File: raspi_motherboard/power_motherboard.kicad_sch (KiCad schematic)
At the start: 20 parts, among them J1 GPIO, J2 Conn_02x04_Top_Bottom

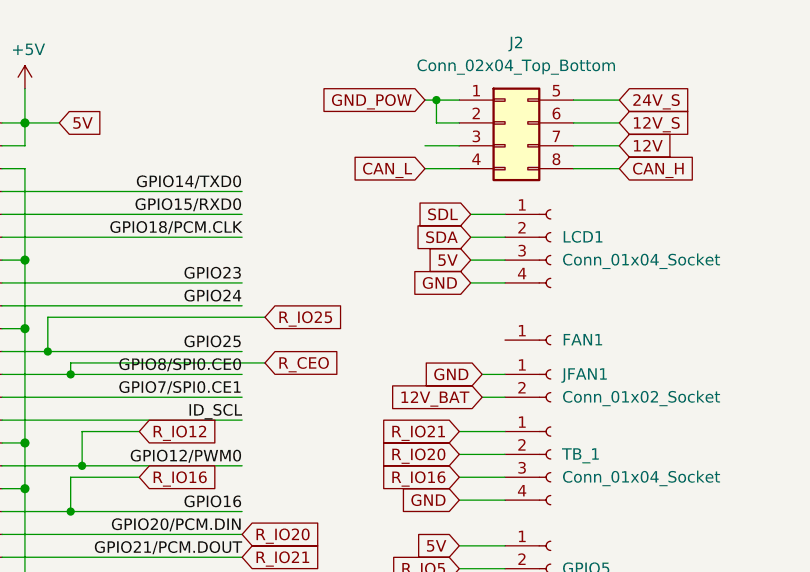
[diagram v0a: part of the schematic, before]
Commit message: Routed
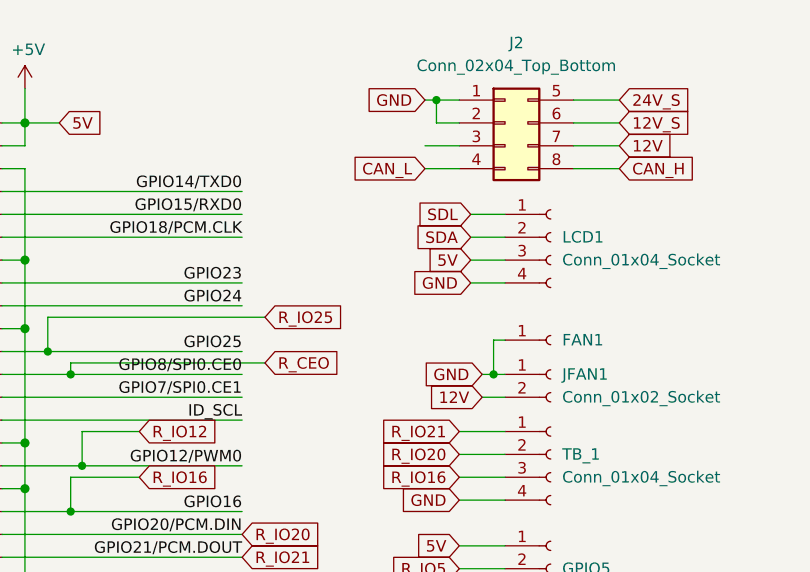
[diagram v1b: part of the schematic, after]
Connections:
- net 12V_BAT is gone; now on net 12V: JFAN1.2 (Pin_2)
- net GND_POW is gone; now on net GND: J2.1 (Pin_1), J2.2 (Pin_2)
- net GND: now also FAN1.1 (Pin_1)
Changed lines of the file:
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@@
+	)
+	(junction
+		(at 128.27 55.88)
+		(diameter 0)
+		(color 0 0 0 0)
 	)
 	(junction
@@
 	(wire
 		(pts
+			(xy 128.27 52.07) (xy 129.54 52.07)
+		)
+		(stroke
+			(width 0)
+			(type default)
+		)
+	)
+	(wire
+		(pts
 			(xy 124.46 100.33) (xy 129.54 100.33)
 		)
@@
 	(wire
 		(pts
+			(xy 128.27 55.88) (xy 128.27 52.07)
+		)
+		(stroke
+			(width 0)
+			(type default)
+		)
+	)
+	(wire
+		(pts
 			(xy 31.75 45.72) (xy 60.96 45.72)
 		)
@@
 	(wire
 		(pts
+			(xy 128.27 55.88) (xy 129.54 55.88)
+		)
+		(stroke
+			(width 0)
+			(type default)
+		)
+	)
+	(wire
+		(pts
 			(xy 121.92 25.4) (xy 124.46 25.4)
 		)
@@
 	(wire
 		(pts
-			(xy 127 55.88) (xy 129.54 55.88)
+			(xy 127 55.88) (xy 128.27 55.88)
 		)
 		(stroke
@@
 		)
 	)
-	(global_label "12V_BAT"
+	(global_label "12V"
 		(shape input)
 		(at 127 58.42 180)
@@
 		)
 		(property "Intersheetrefs" "${INTERSHEET_REFS}"
-			(at 116.1183 58.42 0)
+			(at 120.4121 58.42 0)
 			(effects
 				(font
@@
 		)
 	)
-	(global_label "GND_POW"
+	(global_label "GND"
 		(shape input)
 		(at 120.65 25.4 180)
@@
 		)
 		(property "Intersheetrefs" "${INTERSHEET_REFS}"
-			(at 108.6797 25.4 0)
-			(effects
-				(font
+			(at 113.6992 25.4 0)
+			(effects
+				(font
